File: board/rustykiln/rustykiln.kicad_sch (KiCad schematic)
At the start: 14 parts, among them IC1 TPS5450DDA, J1 MPM-15-24, U1 RP2040_Stamp

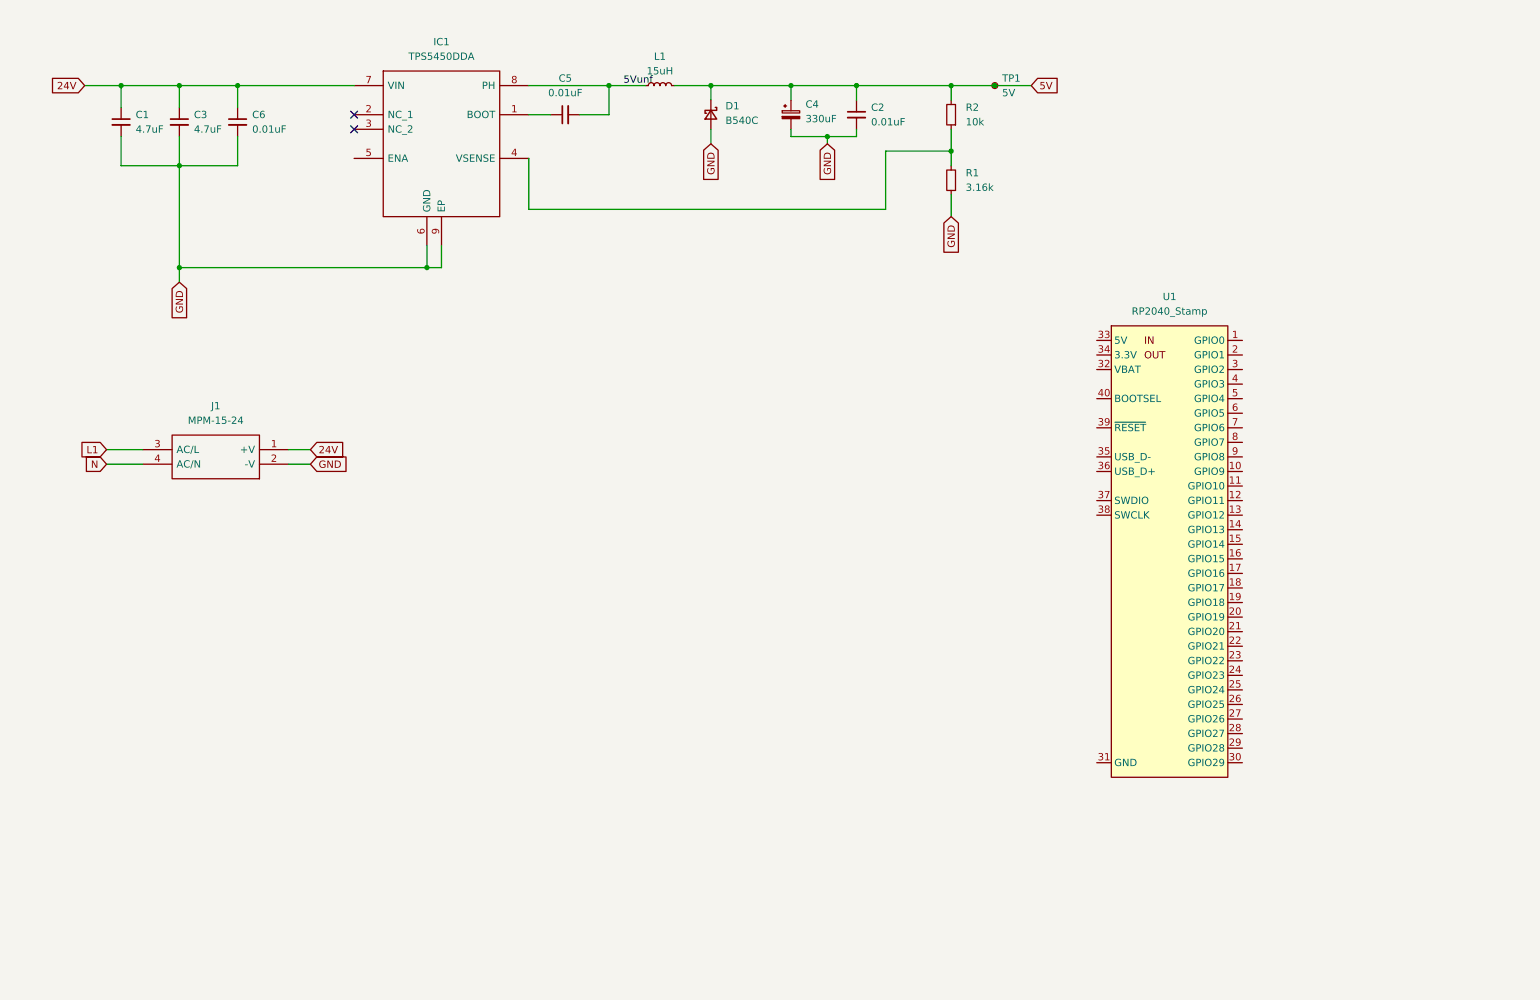
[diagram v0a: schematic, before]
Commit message: Updates
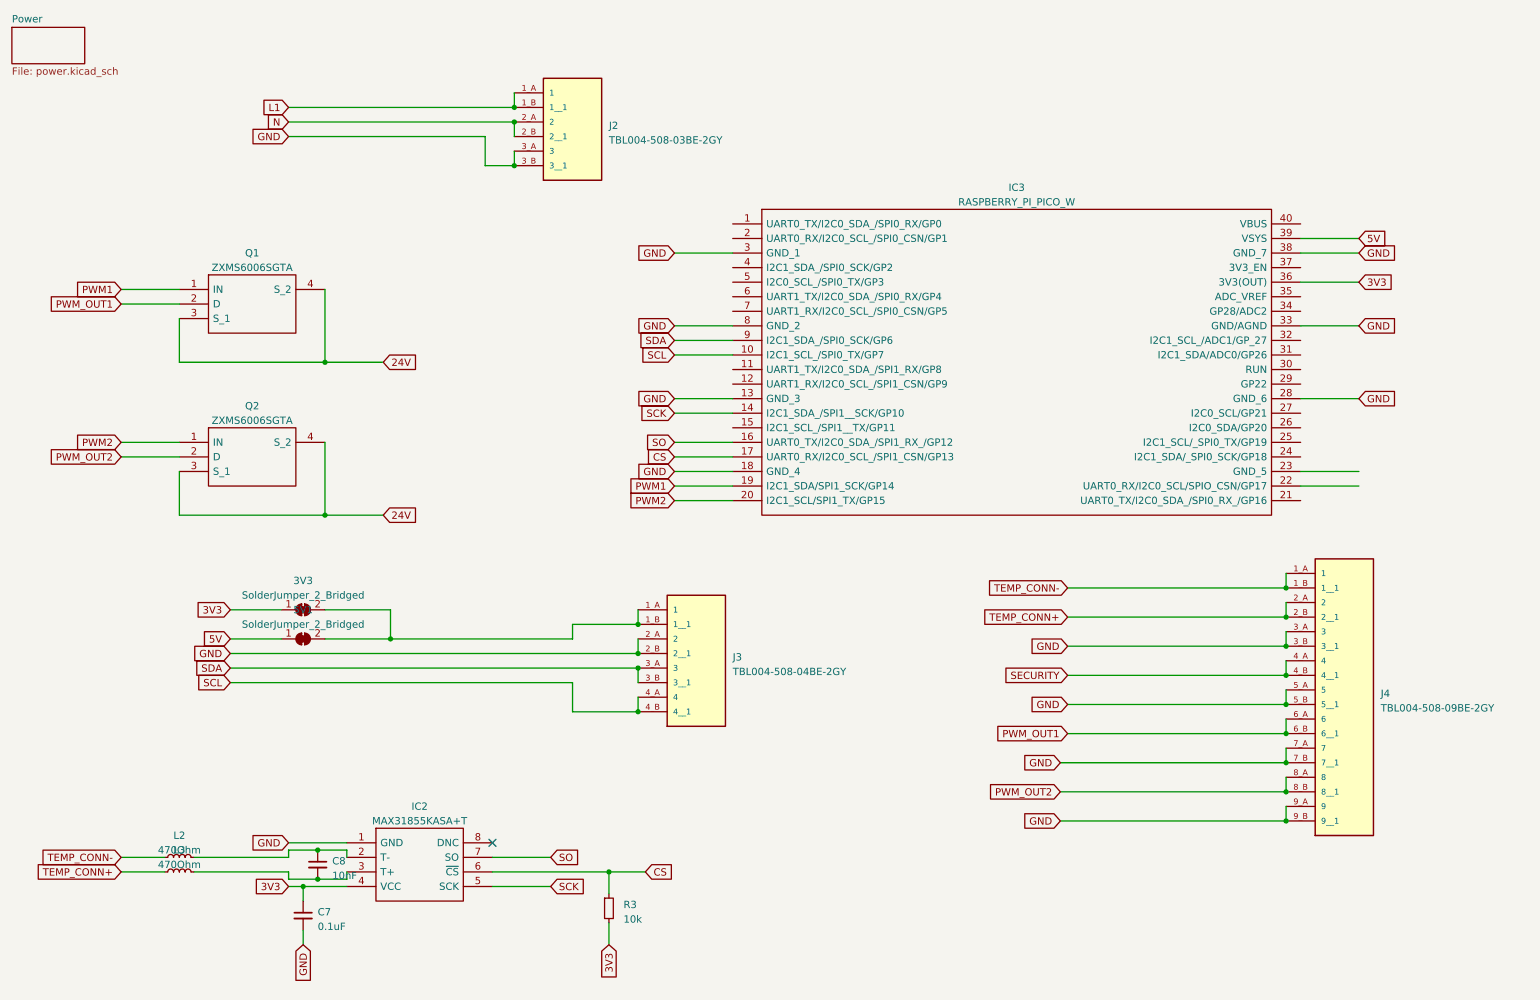
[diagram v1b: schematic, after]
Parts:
- removed C1, C3: 4.7uF, Capacitor_SMD:C_0805_2012Metric, symbol Device:C_Small
- removed C2, C5, C6: 0.01uF, Capacitor_SMD:C_0805_2012Metric, symbol Device:C_Small
- removed C4: 330uF, SamacSys_Parts:POSCAP_D12_D15_D15E_D2E_D2_D3L_D4, symbol Device:C_Polarized_Small
- removed D1: B540C, SamacSys_Parts:DIOM7959X250N, symbol Device:D_Schottky_Small
- removed IC1: TPS5450DDA, SamacSys_Parts:SOIC127P600X170-9N, symbol SamacSys_Parts:TPS5450DDA
- removed J1: MPM-15-24, SamacSys_Parts:MPM1524, symbol SamacSys_Parts:MPM-15-24
- removed L1: 15uH, SamacSys_Parts:INDPM120120X800N, symbol Device:L_Small
- removed R1: 3.16k, Resistor_SMD:R_0805_2012Metric, symbol Device:R_Small
- removed R2: 10k, Resistor_SMD:R_0805_2012Metric, symbol Device:R_Small
- removed TP1: 5V, TestPoint:TestPoint_Pad_D1.5mm, symbol Connector:TestPoint_Small
- removed U1: RP2040_Stamp, RP2040:RP2040_Stamp_SMD, symbol RP2040_Stamp:RP2040_Stamp
- added 3V3, 5V1: SolderJumper_2_Bridged, Jumper:SolderJumper-2_P1.3mm_Bridged_RoundedPad1.0x1.5mm, symbol Jumper:SolderJumper_2_Bridged
- added C7: 0.1uF, Capacitor_SMD:C_0402_1005Metric_Pad0.74x0.62mm_HandSolder, symbol Device:C_Small
- added C8: 10nF, Capacitor_SMD:C_0402_1005Metric_Pad0.74x0.62mm_HandSolder, symbol Device:C_Small
- added IC2: MAX31855KASA+T, libs:SOIC127P600X175-8N, symbol Samacsys:MAX31855KASA+T
- added IC3: RASPBERRY_PI_PICO_W, libs:RASPBERRYPIPICOW, symbol Samacsys:RASPBERRY_PI_PICO_W
- added J2: TBL004-508-03BE-2GY, CUI_TBL004-508-03BE-2GY, symbol TBL004-508-03BE-2GY:TBL004-508-03BE-2GY
- added J3: TBL004-508-04BE-2GY, CUI_TBL004-508-04BE-2GY, symbol TBL004-508-04BE-2GY:TBL004-508-04BE-2GY
- added J4: TBL004-508-09BE-2GY, CUI_TBL004-508-09BE-2GY, symbol TBL004-508-09BE-2GY:TBL004-508-09BE-2GY
- added L2, L3: 470Ohm, Inductor_SMD:L_0603_1608Metric_Pad1.05x0.95mm_HandSolder, symbol Device:L_Small
- added Q1, Q2: ZXMS6006SGTA, libs:SOT230P700X170-4N, symbol Samacsys:ZXMS6006SGTA
- added R3: 10k, Resistor_SMD:R_0603_1608Metric_Pad0.98x0.95mm_HandSolder, symbol Device:R_Small
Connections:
- net 24V: now also Q1.3 (S_1), Q1.4 (S_2), Q2.3 (S_1), Q2.4 (S_2)
- net 5V: now also 5V1.1 (A), IC3.39 (VSYS)
- net GND: now also C7.2, IC2.1 (GND), IC3.13 (GND_3), IC3.18 (GND_4), IC3.28 (GND_6), IC3.3 (GND_1), IC3.33 (GND/AGND), IC3.38 (GND_7), IC3.8 (GND_2), J2.3_A (3), J2.3_B (3__1), J3.2_A (2), J3.2_B (2__1), J4.3_A (3), J4.3_B (3__1), J4.5_A (5), J4.5_B (5__1), J4.7_A (7), J4.7_B (7__1), J4.9_A (9), J4.9_B (9__1)
- net L1: now also J2.1_A (1), J2.1_B (1__1)
- net N: now also J2.2_A (2), J2.2_B (2__1)
- new net: C8.2, IC2.3 (T+), L3.2
- new net: 3V3.2 (B), 5V1.2 (B), J3.1_A (1), J3.1_B (1__1)
- new net: C8.1, IC2.2 (T-), L2.2
- new net 3V3: 3V3.1 (A), C7.1, IC2.4 (VCC), IC3.36 (3V3(OUT)), R3.2
- new net CS: IC2.6 (~{CS}), IC3.17 (UART0_RX/I2C0_SCL_/SPI1_CSN/GP13), R3.1
- new net PWM1: IC3.19 (I2C1_SDA/SPI1_SCK/GP14), Q1.1 (IN)
- new net PWM2: IC3.20 (I2C1_SCL/SPI1_TX/GP15), Q2.1 (IN)
- new net PWM_OUT1: J4.6_A (6), J4.6_B (6__1), Q1.2 (D)
- new net PWM_OUT2: J4.8_A (8), J4.8_B (8__1), Q2.2 (D)
- new net SCK: IC2.5 (SCK), IC3.14 (I2C1_SDA_/SPI1__SCK/GP10)
- new net SCL: IC3.10 (I2C1_SCL_/SPI0_TX/GP7), J3.4_A (4), J3.4_B (4__1)
- new net SDA: IC3.9 (I2C1_SDA_/SPI0_SCK/GP6), J3.3_A (3), J3.3_B (3__1)
- new net SECURITY: J4.4_A (4), J4.4_B (4__1)
- new net SO: IC2.7 (SO), IC3.16 (UART0_TX/I2C0_SDA_/SPI1_RX_/GP12)
- new net TEMP_CONN+: J4.2_A (2), J4.2_B (2__1), L3.1
- new net TEMP_CONN-: J4.1_A (1), J4.1_B (1__1), L2.1
- no-connect marks 2 -> 1
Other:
- added sheet Power (power.kicad_sch)
